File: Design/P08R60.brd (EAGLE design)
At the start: 28 x 26.7 mm, 28 parts, among them P1 PENTABIT_17.32, U1 STM32F091CBU6, U2 VL53L0X, X1 XTALL_CSTCE8M00G52

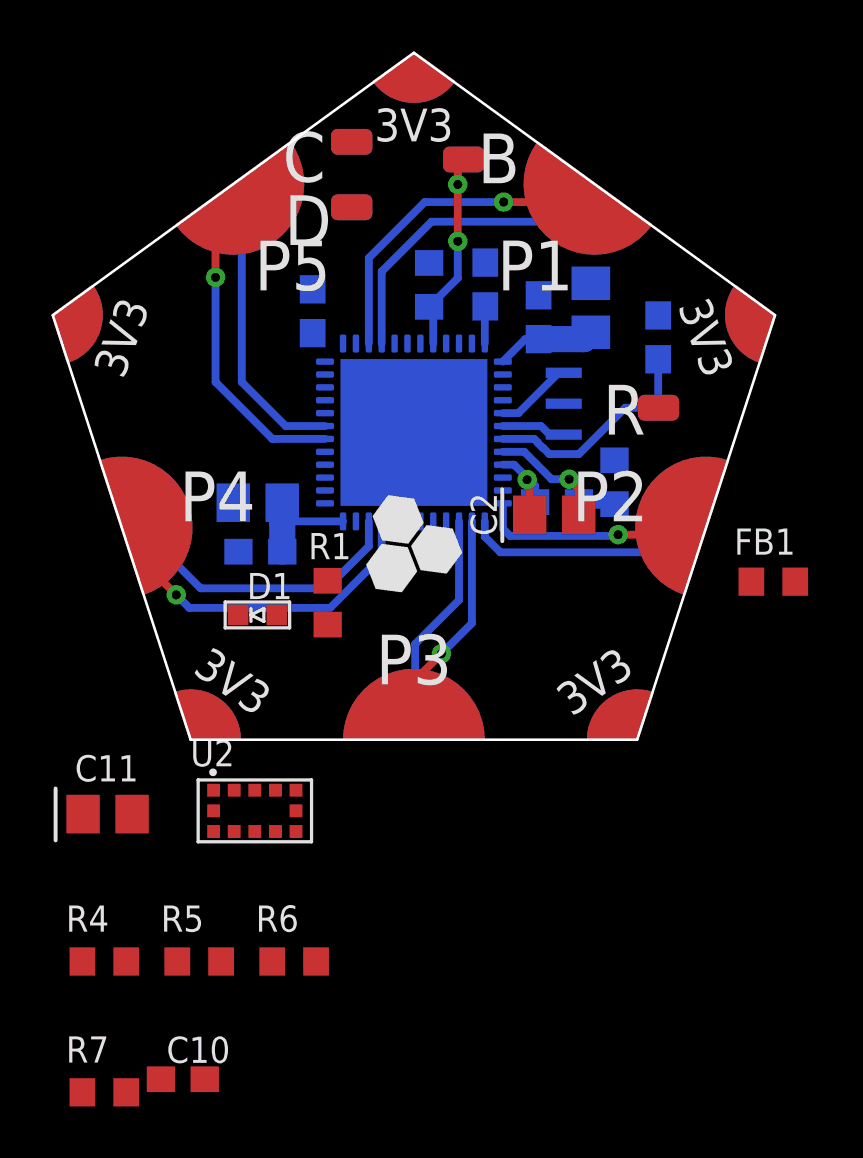
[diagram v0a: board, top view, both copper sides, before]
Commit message: Module ready for Rev 0 release
Finish routing the module
Generate output files
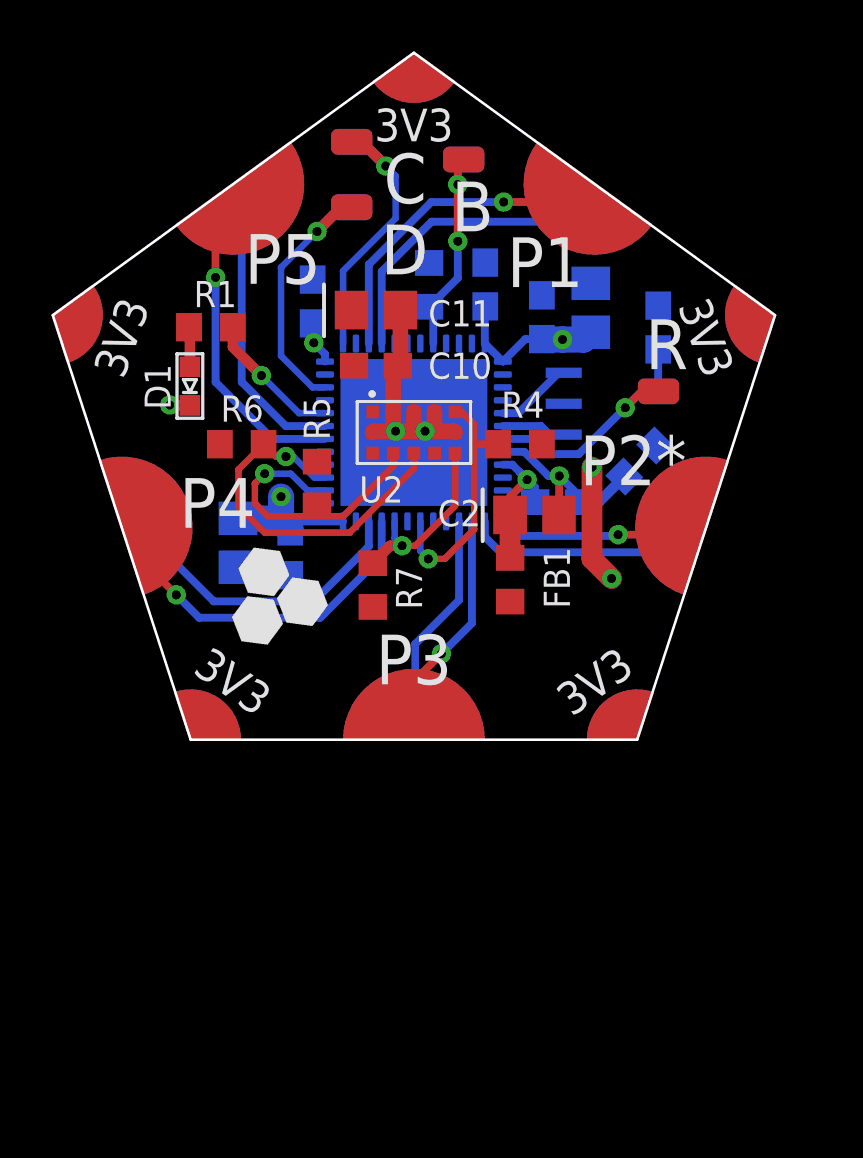
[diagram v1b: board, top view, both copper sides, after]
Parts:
- moved C10 28.7 mm to (33.1, 37.2)
- moved R4 25.7 mm to (38.7, 34.2)
- moved R7 22.3 mm to (33.0, 28.7), turned to 270 degrees
- moved C11 22.2 mm to (33.1, 39.4)
- moved R6 20.2 mm to (27.9, 34.2), turned to 180 degrees
- moved R5 19.1 mm to (30.9, 32.6), turned to 90 degrees
- moved U2 15.9 mm to (34.6, 34.6)
- moved R1 11.6 mm to (26.7, 38.7), turned to 0 degrees
- moved FB1 10.2 mm to (38.4, 28.9), turned to 270 degrees
- moved D1 9.26 mm to (25.9, 36.4), turned to 0 degrees
- moved C4 1.74 mm to (27.8, 30.3), turned to 270 degrees
- moved R2 1.28 mm to (43.4, 33.5), turned to 315 degrees
- moved C6 1.16 mm to (29.8, 29.9), turned to 270 degrees
- moved C2 0.76 mm to (39.3, 31.4)
- moved R 0.63 mm to (44.1, 36.2)
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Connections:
- removed net AGND: C10.2, C11.2, U2.12, U2.2, U2.3, U2.4, U2.6
- net GND: now also C10.2, C11.2, U1.P$16, U1.P$17, U1.P$33, U1.P$41, U1.P$42, U1.P$43, U2.12, U2.2, U2.3, U2.4, U2.6
- net XSHUT: now also U1.P$18; no longer U1.P$25
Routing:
- net GND: track 0.00 -> 15.0 mm, vias 0 -> 5
- net I2C2_SDA: track 0.00 -> 14.6 mm, vias 0 -> 1
- net N$9: track 0.00 -> 11.3 mm, vias 0 -> 1
- net I2C2_SCL: track 0.00 -> 11.2 mm, vias 0 -> 1
- net N$7: track 0.00 -> 11.1 mm, vias 0 -> 1
- net XSHUT: track 0.00 -> 9.77 mm, vias 0 -> 1
- net INT: track 0.00 -> 7.23 mm, vias 0 -> 1
- net N$3: track 0.00 -> 5.41 mm, vias 0 -> 1
- net VDD: track 9.62 -> 14.3 mm, vias 0 -> 3
- net VDDA: track 3.64 -> 5.50 mm
- net R1: track 8.93 -> 10.5 mm, vias 0 -> 1
- net N$4: track 0.00 -> 1.55 mm
- net VSSA: track 7.01 -> 7.60 mm
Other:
- board text added: "P2*"
- board text removed: "P2"
